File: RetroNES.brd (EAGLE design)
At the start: 50.8 x 37.3 mm, 8 parts, among them IC1 ATMEGA32U4-AU

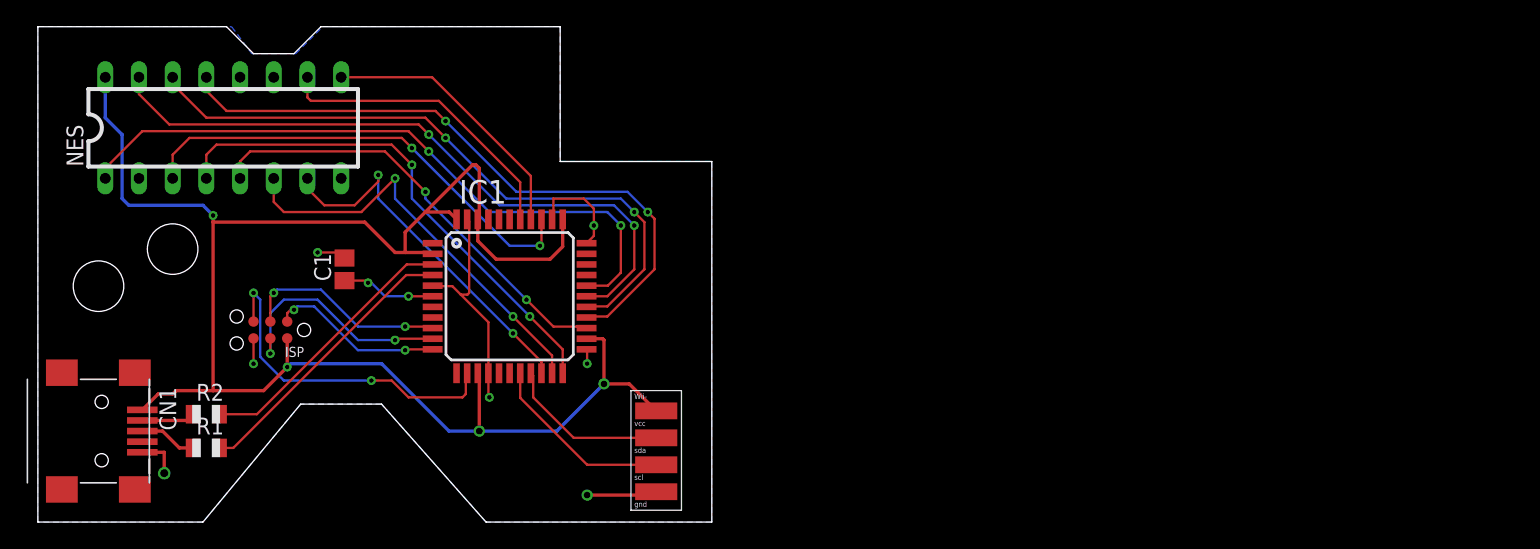
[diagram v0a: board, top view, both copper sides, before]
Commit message: First commit
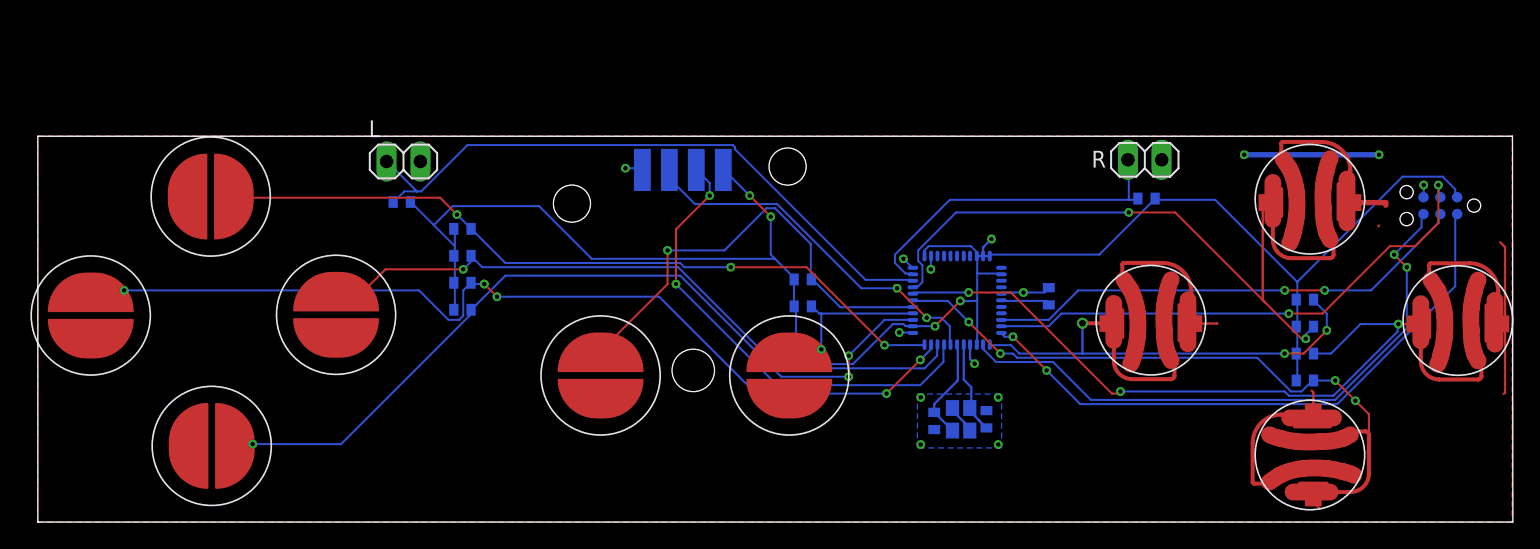
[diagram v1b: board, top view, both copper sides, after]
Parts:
- removed CN1: (no value), adafruit:USB-MINIB
- removed IC1: ATMEGA32U4-AU, adafruit:TQFP44
- removed NES: NES_SOCKET, RetroNES:DIL16
- added A-BUTTON, B-BUTTON, X-BUTTON, Y-BUTTON: AB, NES:A-B
- added C2: 8pf, adafruit:C0402
- added C3: 8pF, adafruit:C0402
- added DOWN-BUTTON, LEFT-BUTTON, RIGHT-BUTTON, SELECT-BUTTON, START-BUTTON, UP-BUTTON: DPAD-SS, NES:DPAD-SS
- added L, R: (no value), pinhead:1X02
- added R10, R11, R12, R3, R4, R5, R6, R7, R8, R9: 1k, adafruit:R0402
- added U$1: ATMEGA32U41:1-LESS_PASTE, SparkFun-DigitalIC:QFN-44-NOPAD_1:1-LESS_PASTE
- added U$2: CX2520DB, adamtemp:2.5MMX2.0MM
- C1: device adafruit:C0805 -> adafruit:C0402
- R1, R2: value 22 -> 1k; device adafruit:R0805 -> adafruit:R0402
- moved ISP 88.7 mm to (105.7, 23.9), flipped to the bottom, turned to 0 degrees
- moved R1 83.6 mm to (95.5, 16.8), flipped to the bottom
- moved R2 83.1 mm to (95.5, 14.7), flipped to the bottom
- moved C1 53.1 mm to (76.2, 17.0), flipped to the bottom
- moved WII 18.9 mm to (50.0, 24.9), flipped to the bottom, turned to 0 degrees
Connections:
- removed net CLOCK: IC1.38, NES.10
- removed net D+: CN1.D+, R1.1
- removed net D+U: IC1.4, R1.2
- removed net D-: CN1.D-, R2.1
- removed net D-U: IC1.3, R2.2
- removed net DO: IC1.36, NES.3
- removed net LATCH: IC1.37, NES.9
- new net L: L.1, R11.1, U$1.31
- new net R: R.1, R12.1, U$1.32
- new net X: R2.1, U$1.30, X-BUTTON.P$1
- new net XTAL1: C3.1, U$1.17, U$2.P$1
- new net XTAL2: C2.1, U$1.16, U$2.P$3
- new net Y: R1.1, U$1.12, Y-BUTTON.P$1
- net A: now also A-BUTTON.P$1, R10.1, U$1.29; no longer IC1.29, NES.1
- net B: now also B-BUTTON.P$1, R9.1, U$1.28; no longer IC1.28, NES.15
- net DOWN: now also DOWN-BUTTON.P$1, R5.1, U$1.25; no longer IC1.25, NES.5
- net GND: now also A-BUTTON.P$2, B-BUTTON.P$2, C2.2, C3.2, DOWN-BUTTON.P$2, L.2, LEFT-BUTTON.P$2, R.2, RIGHT-BUTTON.P$2, SELECT-BUTTON.P$2, START-BUTTON.P$2, U$1.15, U$1.23, U$1.33, U$1.35, U$1.43, U$1.5, U$2.P$2, U$2.P$4, UP-BUTTON.P$2, X-BUTTON.P$2, Y-BUTTON.P$2; no longer CN1.GND, IC1.15, IC1.23, IC1.33, IC1.35, IC1.43, IC1.5, NES.11, NES.8
- net LEFT: now also LEFT-BUTTON.P$1, R6.1, U$1.21; no longer IC1.21, NES.6
- net MISO: now also U$1.11; no longer IC1.11
- net MOSI: now also U$1.10; no longer IC1.10
- net RESET: now also U$1.13; no longer IC1.13
- net RIGHT: now also R4.1, RIGHT-BUTTON.P$1, U$1.20; no longer IC1.20, NES.7
- net SCK: now also U$1.9; no longer IC1.9
- net SCL: now also U$1.18; no longer IC1.18
- net SDA: now also U$1.19; no longer IC1.19
- net SELECT: now also R7.1, SELECT-BUTTON.P$1, U$1.27; no longer IC1.27, NES.14
- net START: now also R8.1, START-BUTTON.P$1, U$1.26; no longer IC1.26, NES.13
- net UCAP: now also U$1.6; no longer IC1.6
- net UP: now also R3.1, U$1.22, UP-BUTTON.P$1; no longer IC1.22, NES.4
- net VCC: now also R1.2, R10.2, R11.2, R12.2, R2.2, R3.2, R4.2, R5.2, R6.2, R7.2, R8.2, R9.2, U$1.14, U$1.2, U$1.24, U$1.34, U$1.42, U$1.44; no longer CN1.VBUS, IC1.14, IC1.2, IC1.24, IC1.34, IC1.42, IC1.44, NES.16
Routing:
- net L: track 0.00 -> 48.5 mm
- net X: track 0.00 -> 46.5 mm, vias 0 -> 2
- net LEFT: track 31.9 -> 71.7 mm, vias 2 -> 5
- net START: track 49.2 -> 13.0 mm, vias 2 -> 1
- net DO: track 35.4 -> 0.00 mm, vias 2 -> 0
- net Y: track 0.00 -> 33.1 mm, vias 0 -> 3
- net MISO: track 13.2 -> 45.7 mm
- net DOWN: track 34.1 -> 62.3 mm, vias 2 -> 3
- net R: track 0.00 -> 25.5 mm
- net RIGHT: track 27.9 -> 51.5 mm, vias 2 -> 1
- net SDA: track 12.4 -> 35.5 mm, vias 0 -> 2
- net CLOCK: track 23.0 -> 0.00 mm
- net MOSI: track 18.2 -> 40.0 mm
- net D+U: track 21.5 -> 0.00 mm
- net SCK: track 15.6 -> 36.8 mm
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- added copper zone on layer 1, net GND
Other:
- board size 50.8 x 37.3 mm -> 111.2 x 29.1 mm
